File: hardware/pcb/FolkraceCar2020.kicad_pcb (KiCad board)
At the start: 2 copper layers, 100 x 67 mm, 3 parts, among them J2 Jetson Nano Header, U1 TPS25940x-Q1, U2 OKL-T_6-W12N-C

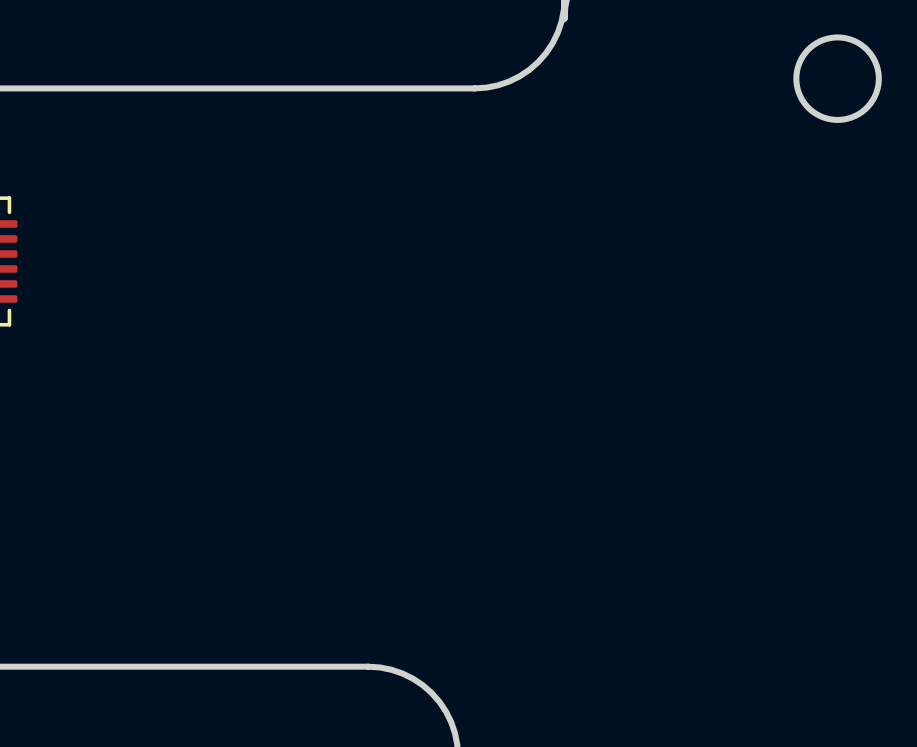
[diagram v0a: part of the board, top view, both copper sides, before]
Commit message: updated schematic
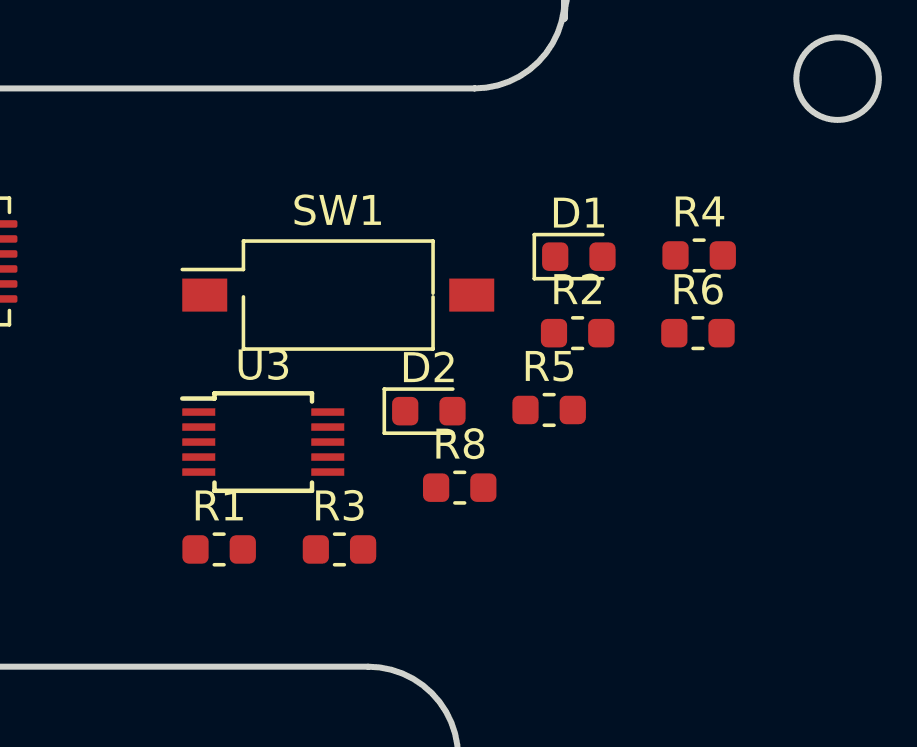
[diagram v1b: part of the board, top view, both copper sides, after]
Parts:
- added D1: LED RED, LED_SMD:LED_0603_1608Metric, F.Cu at (162.5, 87.0)
- added D2: LED GREEN, LED_SMD:LED_0603_1608Metric, F.Cu at (157.5, 92.2)
- added R1: R, Resistor_SMD:R_0603_1608Metric, F.Cu at (150.5, 96.8)
- added R2: R, Resistor_SMD:R_0603_1608Metric, F.Cu at (162.5, 89.5)
- added R3: R, Resistor_SMD:R_0603_1608Metric, F.Cu at (154.5, 96.8)
- added R4: R, Resistor_SMD:R_0603_1608Metric, F.Cu at (166.5, 87.0)
- added R5: R, Resistor_SMD:R_0603_1608Metric, F.Cu at (161.5, 92.1)
- added R6: R, Resistor_SMD:R_0603_1608Metric, F.Cu at (166.5, 89.5)
- added R8: R, Resistor_SMD:R_0603_1608Metric, F.Cu at (158.5, 94.7)
- added SW1: SPST, Button_Switch_SMD:SW_DIP_SPSTx01_Slide_Omron_A6S-110x_W8.9mm_P2.54mm, F.Cu at (154.5, 88.3)
- added U3: ADS1115IDGS, Package_SO:TSSOP-10_3x3mm_P0.5mm, F.Cu at (152.0, 93.2)
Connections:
- U1 pad 16: Net-(U1-Pad16) -> GND
- U1 pad 2: Net-(U1-Pad2) -> Net-(R8-Pad1)
- U1 pad 21: Net-(U1-Pad21) -> GND
- U1 pad 3: Net-(U1-Pad3) -> VBUS
- U1 pad 4: Net-(U1-Pad4) -> VBUS
- U1 pad 5: Net-(U1-Pad5) -> VBUS
- U1 pad 6: Net-(U1-Pad6) -> VBUS
- U1 pad 7: Net-(U1-Pad7) -> VBUS
- U1 pad 8: Net-(U1-Pad8) -> VBUS
- U2 pad 1: Net-(U2-Pad1) -> Net-(R8-Pad1)
- U2 pad 2: Net-(U2-Pad2) -> VBUS
